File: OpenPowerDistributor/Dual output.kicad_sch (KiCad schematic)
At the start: 18 parts, among them J2 Barrel_Jack, Q1 STN2610D, Q2 BC847, Q3 BC847, U3 LM324

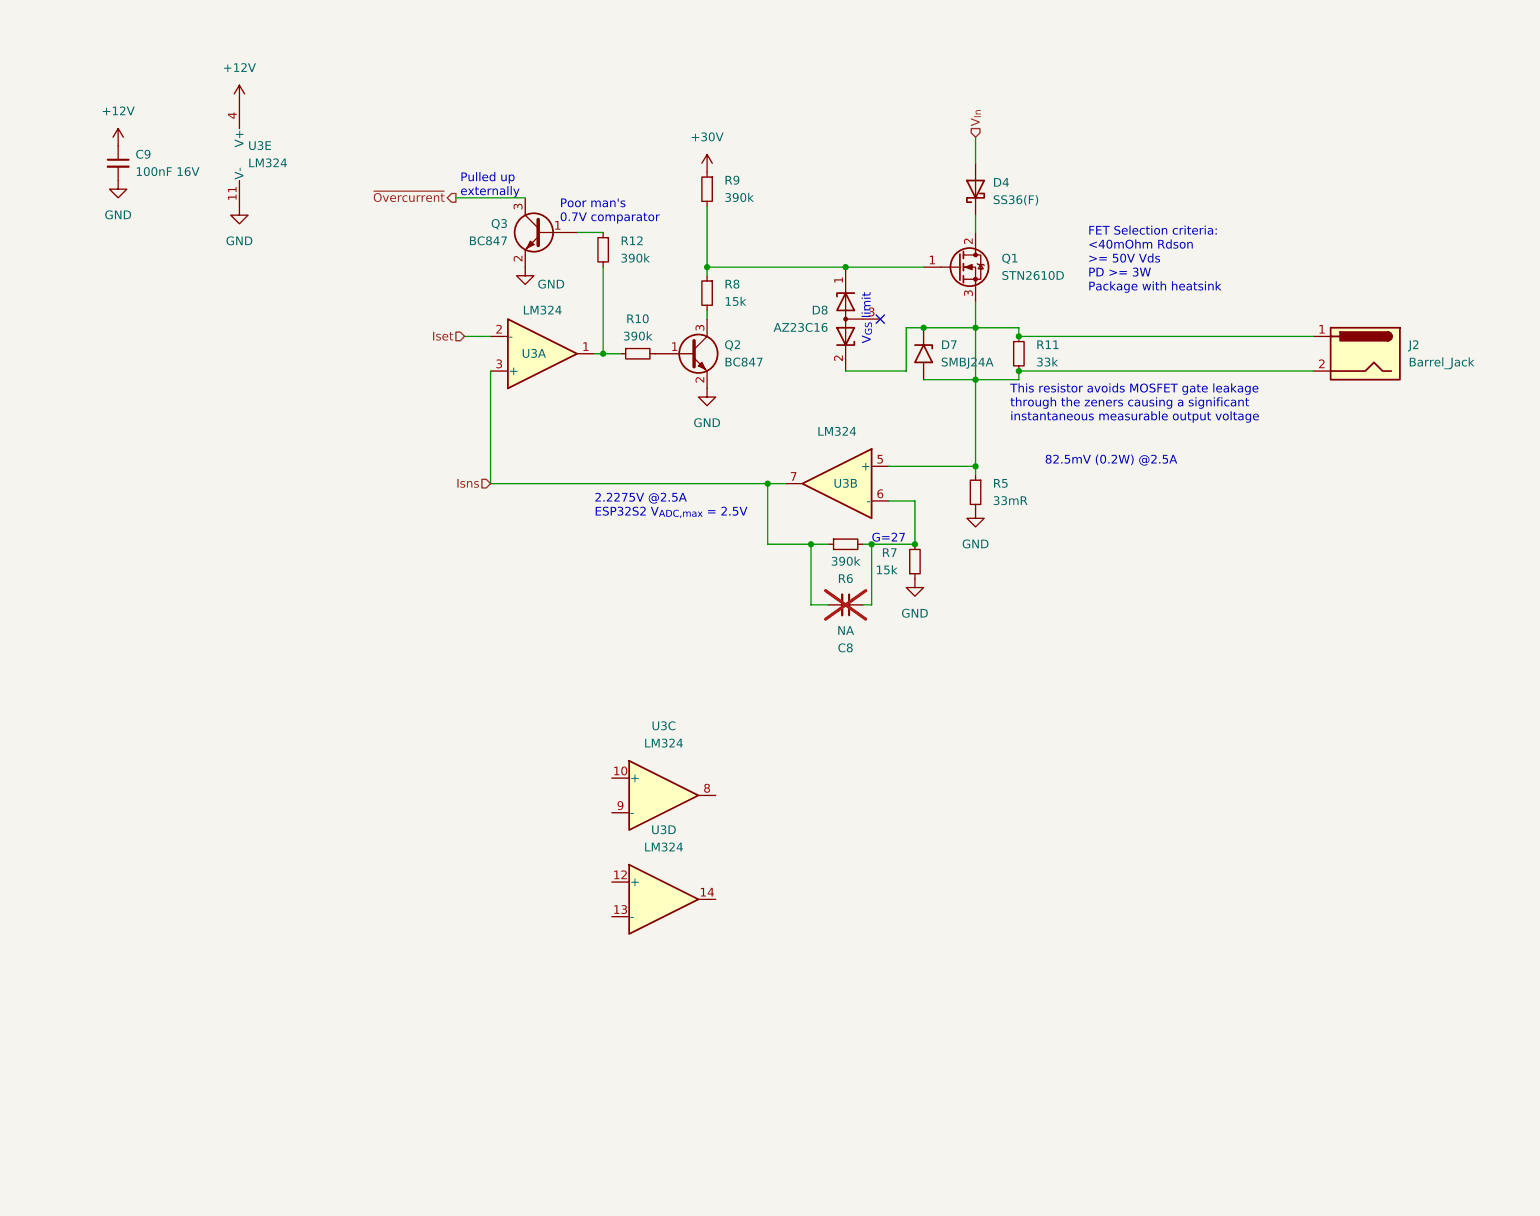
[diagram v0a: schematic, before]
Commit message: More schematic progress
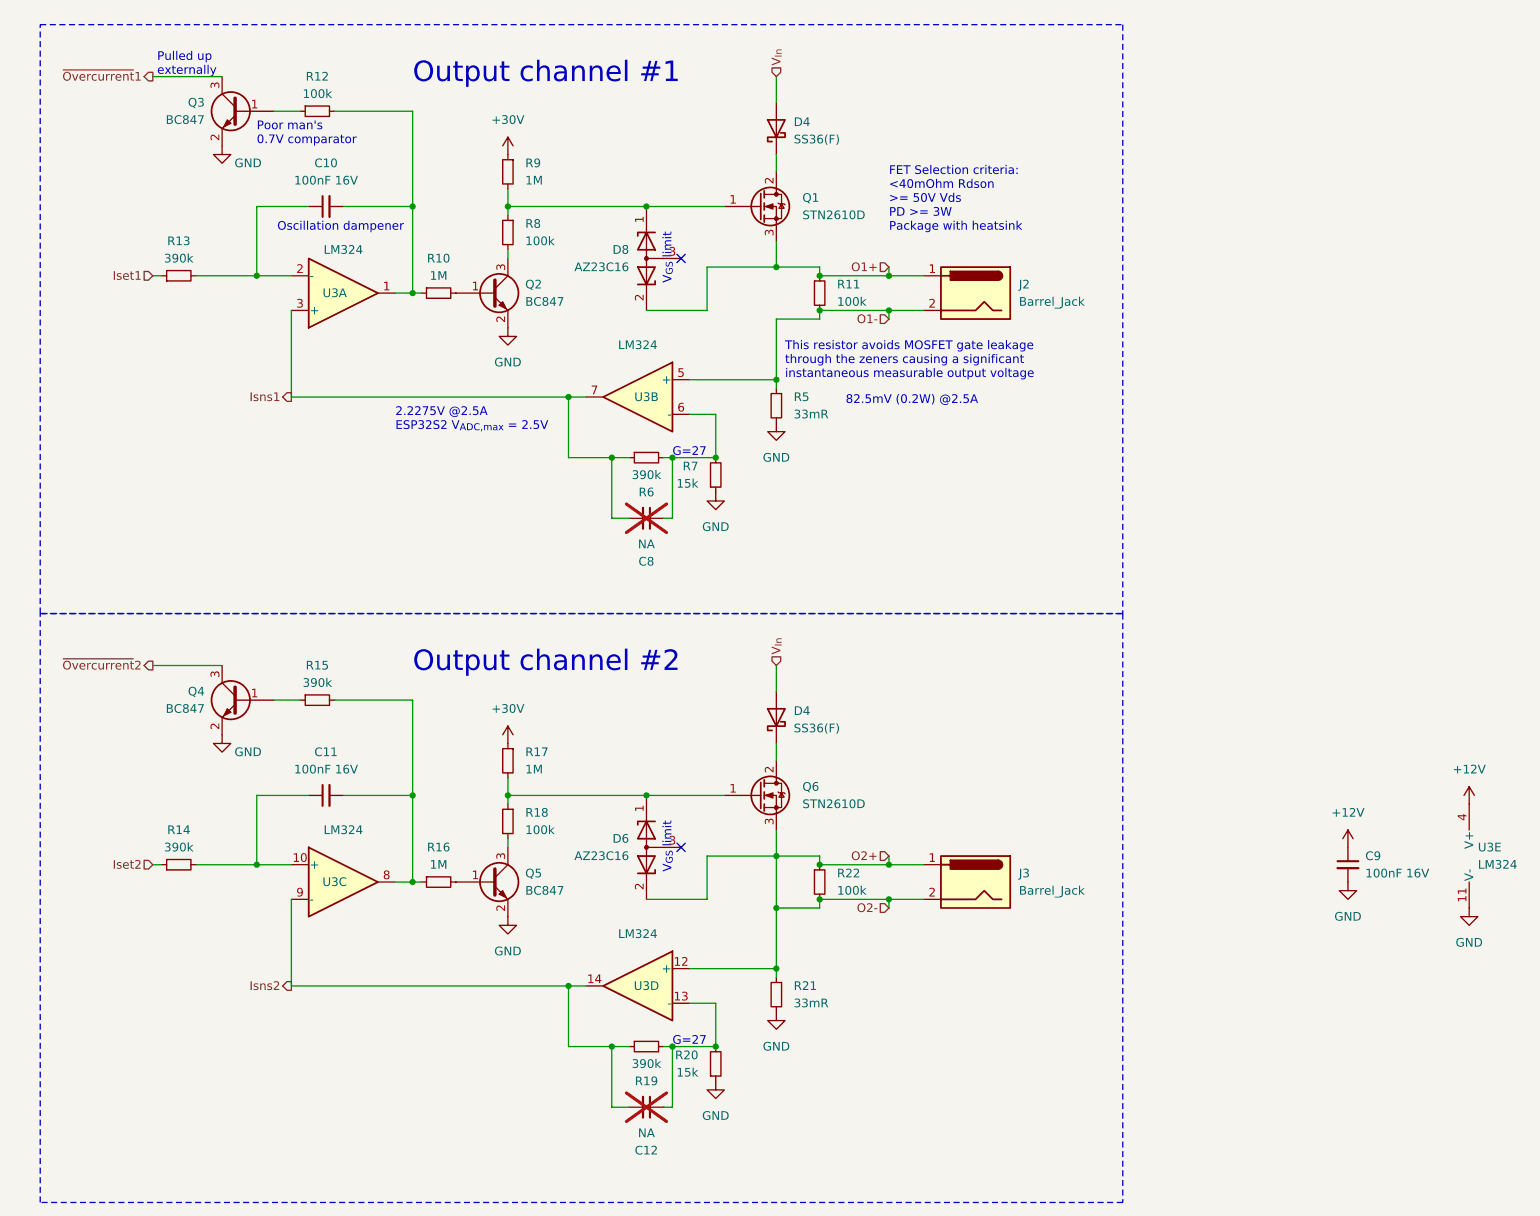
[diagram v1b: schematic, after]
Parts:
- removed D7: SMBJ24A, Diode_SMD:D_SMA, symbol Diode:SMAJ12A
- added C10, C11: 100nF 16V, Capacitor_SMD:C_0603_1608Metric, symbol Device:C_Small
- added C12: NA, Capacitor_SMD:C_0603_1608Metric, symbol Device:C_Small
- added D4: SS36(F), Diode_SMD:D_SMA, symbol Device:D_Schottky
- added D6: AZ23C16, Package_TO_SOT_SMD:SOT-23, symbol Device:D_Zener_Dual_CommonAnode_KKA
- added J3: Barrel_Jack, Connector_BarrelJack:BarrelJack_Horizontal, symbol Connector:Barrel_Jack
- added Q4, Q5: BC847, Package_TO_SOT_SMD:SOT-23, symbol Transistor_BJT:BC847
- added Q6: STN2610D, Package_TO_SOT_SMD:TO-252-2, symbol Transistor_FET:IPD50R3K0CE
- added R13, R14, R15, R19: 390k, Resistor_SMD:R_0603_1608Metric, symbol Device:R_Small
- added R16, R17: 1M, Resistor_SMD:R_0603_1608Metric, symbol Device:R_Small
- added R18, R22: 100k, Resistor_SMD:R_0603_1608Metric, symbol Device:R_Small
- added R20: 15k, Resistor_SMD:R_0603_1608Metric, symbol Device:R_Small
- added R21: 33mR, Resistor_SMD:R_1206_3216Metric, symbol Device:R_Small
- C8: footprint (none) -> Capacitor_SMD:C_0603_1608Metric
- D8: footprint (none) -> Package_TO_SOT_SMD:SOT-23
- J2: footprint (none) -> Connector_BarrelJack:BarrelJack_Horizontal
- R10, R9: value 390k -> 1M; footprint (none) -> Resistor_SMD:R_0603_1608Metric
- R11: value 33k -> 100k; footprint (none) -> Resistor_SMD:R_0603_1608Metric
- R12: value 390k -> 100k; footprint (none) -> Resistor_SMD:R_0603_1608Metric
- R6, R7: footprint (none) -> Resistor_SMD:R_0603_1608Metric
- R8: value 15k -> 100k; footprint (none) -> Resistor_SMD:R_0603_1608Metric
- U3: footprint (none) -> Package_SO:TSSOP-14_4.4x5mm_P0.65mm
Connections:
- net +30V: now also R17.1
- net GND: now also Q4.2 (E), Q5.2 (E), R20.1, R21.2
- net V_{In}: now also D4.2 (A)
- net O1+: now reaches D8.2 (K), J2.1, Q1.3 (S), R11.1
- net O1+: no longer J2.2, R11.2, R5.1, U3.5 (+)
- net at R10.1, R12.2, U3.1: now also C10.2
- net at U3.10 (+): now also C11.1, R14.2
- net at U3.8: now also C11.2, R15.2, R16.1
- net Isns2: now reaches U3.9 (-)
- net Isns2: now also U3.14, C12.2, R19.1
- net O2+: now reaches U3.12 (+)
- net O2+: now also D6.2 (K), J3.1, J3.2, Q6.3 (S), R21.1, R22.1, R22.2
- net at U3.13 (-): now also C12.1, R19.2, R20.2
- net Iset: no longer names the net of U3.2 (-)
- net Iset: now also C10.1, R13.2
- net Isns renamed Isns1
- net ~{Overcurrent} renamed ~{Overcurrent}1
- new net: D6.1 (K), Q6.1 (G), R17.2, R18.1
- new net: Q5.3 (C), R18.2
- new net: D4.1 (K), Q6.2 (D)
- new net: Q5.1 (B), R16.2
- new net: Q4.1 (B), R15.1
- new net Iset1: R13.1
- new net Iset2: R14.1
- new net O1-: J2.2, R11.2, R5.1, U3.5 (+)
- new net ~{Overcurrent}2: Q4.3 (C)
- no-connect marks 1 -> 2
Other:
- note added: "Oscillation dampener"
- note added: "Output channel #1"
- note added: "Output channel #2"
- moved on the sheet: C8, C9, D4, D8, J2, Q1, Q2, Q3, R10, R11, R12, R5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
